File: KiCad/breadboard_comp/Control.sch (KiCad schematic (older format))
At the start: 88 parts, among them SW8 SW_Push, U2 74LS04, U57 74LS04, U85 74LS02, U87 74LS08, U88 74LS161, U89 74LS138, U90 28C256, U91 28C256, U92 74LS04, U93 28C256, U94 28C256, U95 74LS04, U96 74LS04

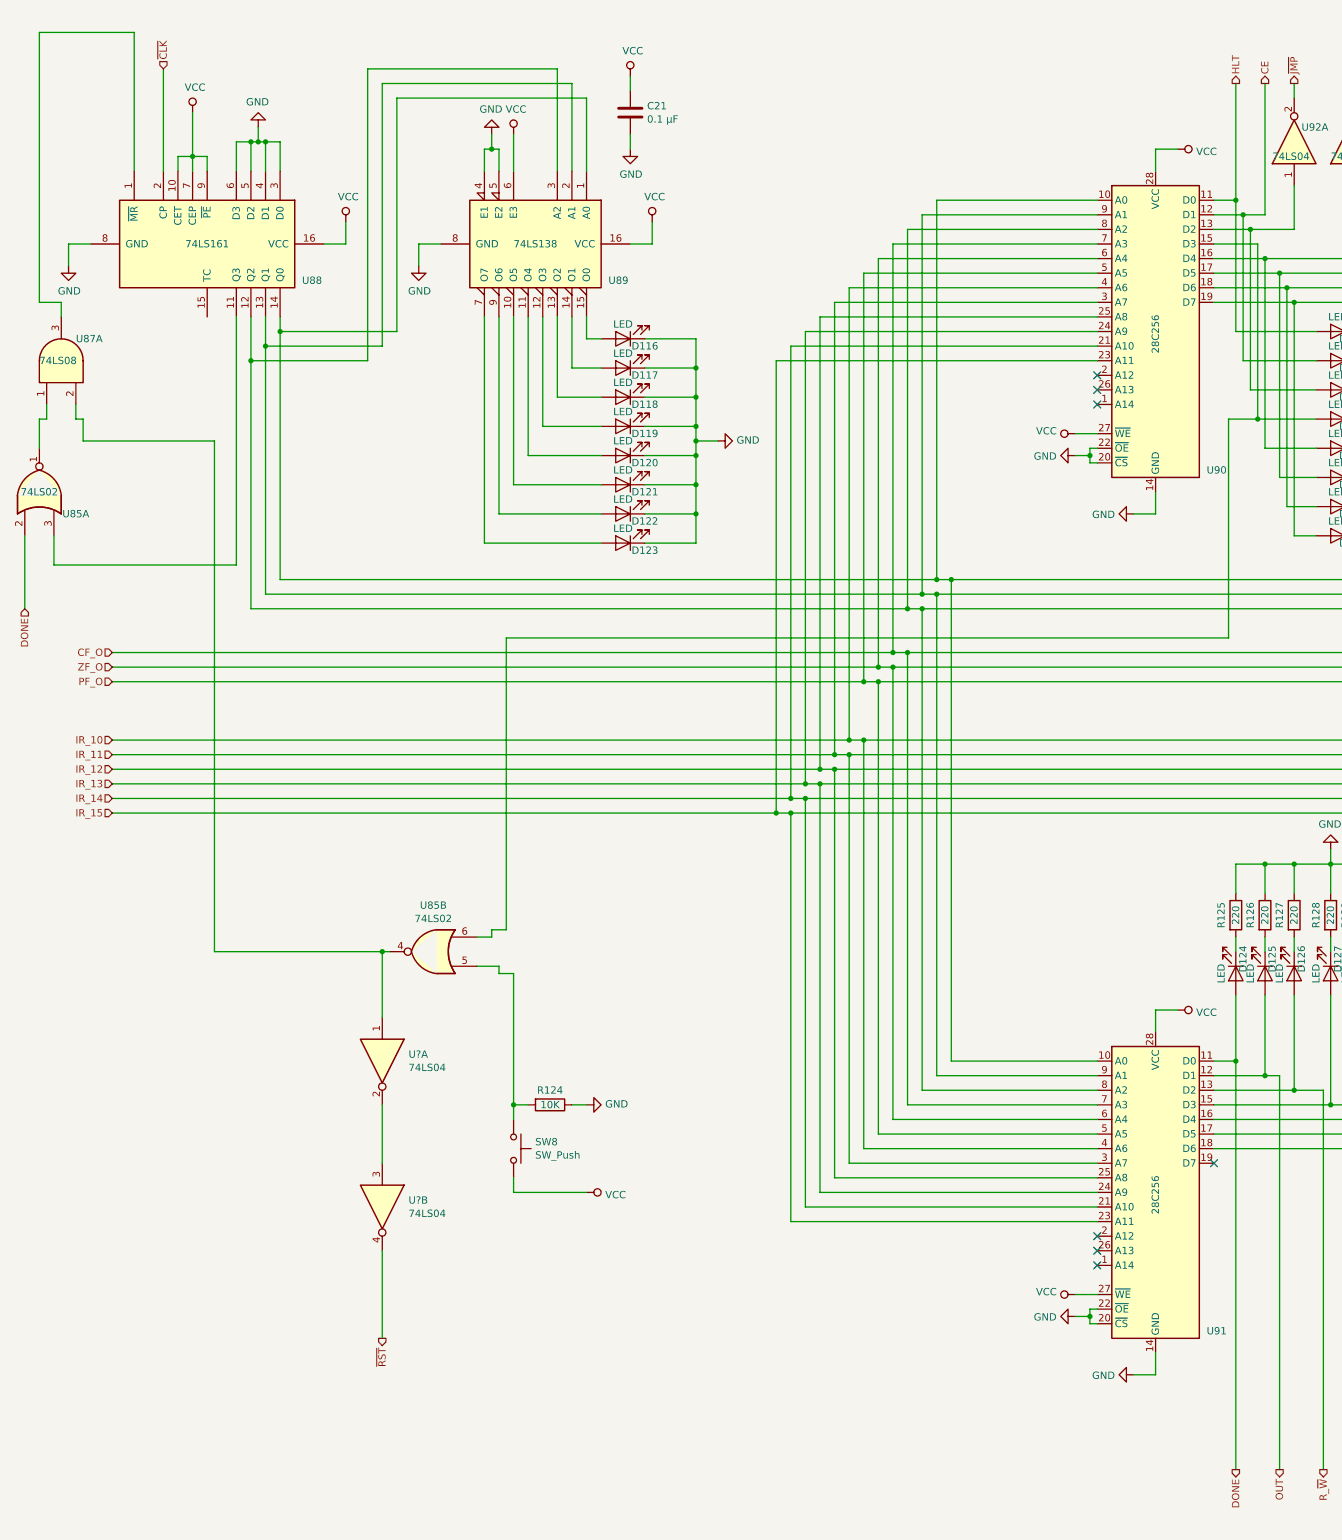
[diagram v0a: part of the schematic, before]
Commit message: Changes
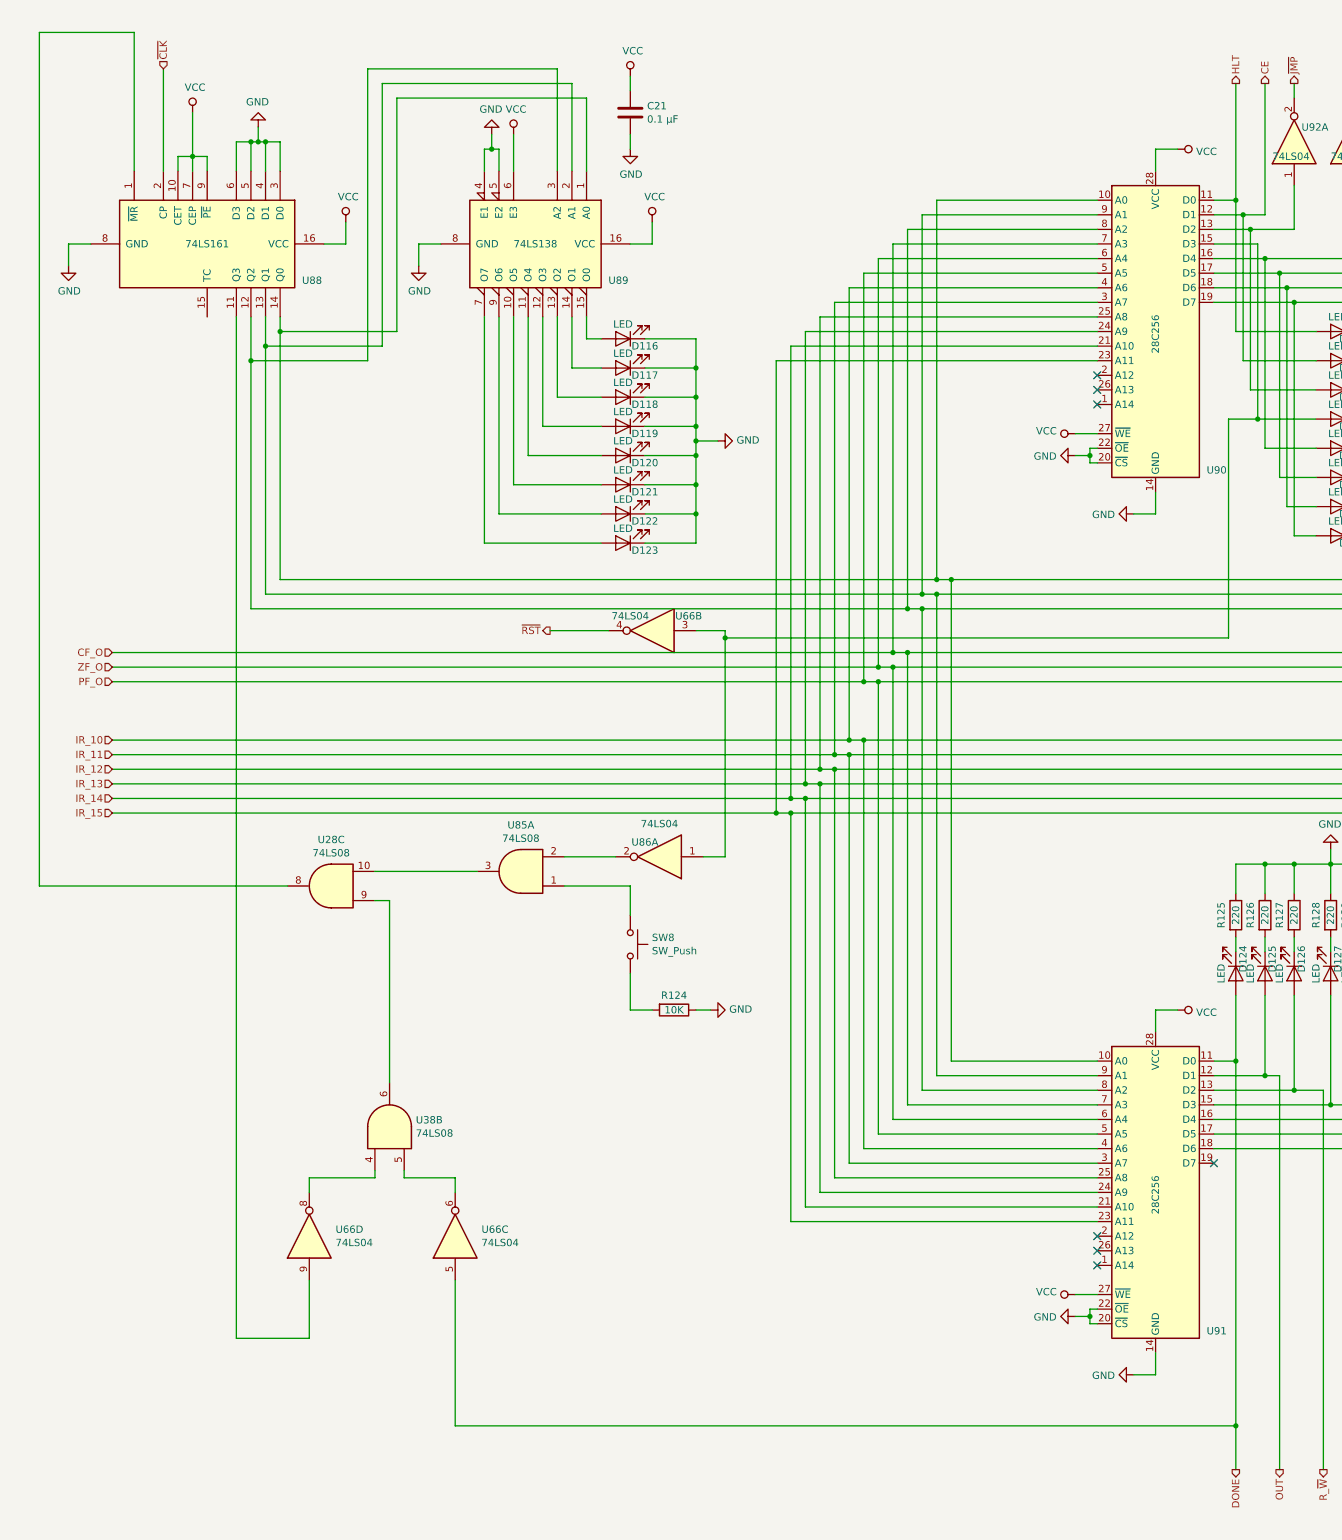
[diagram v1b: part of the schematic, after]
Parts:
- removed U85: 74LS02, symbol 74xx:74LS02
- removed U87: 74LS08, symbol 74xx:74LS08
- removed U? (x2): 74LS04, symbol 74xx:74LS04
- added U28, U38, U85: 74LS08, symbol 74xx:74LS08
- added U66, U86: 74LS04, symbol 74xx:74LS04
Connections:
- net DONE: now also U66.5
- net VCC: no longer SW8.2
- net ~RST: now also U66.4
- net at U88.1 (~MR): now also U28.8
- net at SW8.1: now also U85.1; no longer R124.2
- net at D131.2 (A), U90.15 (D3): now also U66.3, U86.1
- net at U88.11 (Q3): now also U66.9
- new net: R124.2, SW8.2
- new net: U85.2, U86.2
- new net: U28.10, U85.3
- new net: U38.5, U66.6
- new net: U38.4, U66.8
- new net: U28.9, U38.6
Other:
- moved on the sheet: R124, SW8
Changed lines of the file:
@@
 	10250 2450 10250 1650
-$Comp
-L 74xx:74LS08 U87
-U 1 1 5E950B6B
-P 800 2850
-F 0 "U87" V 950 2750 50  0000 R CNN
-F 1 "74LS08" V 800 3000 50  0000 R CNN
-F 2 "" H 800 2850 50  0001 C CNN
-F 3 "http://www.ti.com/lit/gpn/sn74LS08" H 800 2850 50  0001 C CNN
-	1    800  2850
-	0    -1   -1   0
-$EndComp
 $Comp
 L power:GND #PWR0218
@@
 $EndComp
 $Comp
-L 74xx:74LS02 U85
-U 1 1 5F5126B5
-P 650 3750
-F 0 "U85" V 500 3500 50  0000 C CNN
-F 1 "74LS02" V 650 3750 50  0000 C CNN
-F 2 "" H 650 3750 50  0001 C CNN
-F 3 "http://www.ti.com/lit/gpn/sn74ls02" H 650 3750 50  0001 C CNN
-	1    650  3750
-	0    -1   -1   0
-$EndComp
-$Comp
 L Switch:SW_Push SW8
 U 1 1 5E95E647
-P 3900 8250
-F 0 "SW8" V 3854 8398 50  0000 L CNN
-F 1 "SW_Push" V 3945 8398 50  0000 L CNN
-F 2 "" H 3900 8450 50  0001 C CNN
-F 3 "~" H 3900 8450 50  0001 C CNN
-	1    3900 8250
+P 4700 6850
+F 0 "SW8" V 4654 6998 50  0000 L CNN
+F 1 "SW_Push" V 4745 6998 50  0000 L CNN
+F 2 "" H 4700 7050 50  0001 C CNN
+F 3 "~" H 4700 7050 50  0001 C CNN
+	1    4700 6850
 	0    1    1    0
 $EndComp
@@
 L Device:R R124
 U 1 1 5E95EEBA
-P 4150 7950
-F 0 "R124" V 4050 7950 50  0000 C CNN
-F 1 "10K" V 4150 7950 50  0000 C CNN
-F 2 "" V 4080 7950 50  0001 C CNN
-F 3 "~" H 4150 7950 50  0001 C CNN
-	1    4150 7950
-	0    1    1    0
-$EndComp
-Wire Wire Line
-	3900 8550 3900 8450
-$Comp
-L power:VCC #PWR0219
-U 1 1 5E98986A
-P 4400 8550
-F 0 "#PWR0219" H 4400 8400 50  0001 C CNN
-F 1 "VCC" V 4417 8678 50  0000 L CNN
-F 2 "" H 4400 8550 50  0001 C CNN
-F 3 "" H 4400 8550 50  0001 C CNN
-	1    4400 8550
+P 5000 7300
+F 0 "R124" V 4900 7300 50  0000 C CNN
+F 1 "10K" V 5000 7300 50  0000 C CNN
+F 2 "" V 4930 7300 50  0001 C CNN
+F 3 "~" H 5000 7300 50  0001 C CNN
+	1    5000 7300
 	0    1    1    0
 $EndComp
@@
 L power:GND #PWR0220
 U 1 1 5E99EF31
-P 4400 7950
-F 0 "#PWR0220" H 4400 7700 50  0001 C CNN
-F 1 "GND" V 4405 7822 50  0000 R CNN
-F 2 "" H 4400 7950 50  0001 C CNN
-F 3 "" H 4400 7950 50  0001 C CNN
-	1    4400 7950
-	0    -1   -1   0
-$EndComp
-Wire Wire Line
-	4400 7950 4300 7950
-Wire Wire Line
-	650  3450 650  3250
-Wire Wire Line
-	650  3250 700  3250
-Wire Wire Line
-	700  3250 700  3150
-Wire Wire Line
-	800  2550 800  2450
-Wire Wire Line
-	800  2450 650  2450
-Wire Wire Line
-	650  600  650  2450
-Wire Wire Line
-	750  4050 750  4250
-Wire Wire Line
-	750  4250 2000 4250
-Wire Wire Line
-	2000 2550 2000 4250
+P 5250 7300
+F 0 "#PWR0220" H 5250 7050 50  0001 C CNN
+F 1 "GND" V 5255 7172 50  0000 R CNN
+F 2 "" H 5250 7300 50  0001 C CNN
+F 3 "" H 5250 7300 50  0001 C CNN
+	1    5250 7300
+	0    -1   -1   0
+$EndComp
+Wire Wire Line
+	5250 7300 5150 7300
 Text HLabel 15450 950  1    50   Output ~ 0
 ~AO
@@
 	8700 7650 8850 7650
 Wire Wire Line
-	8850 7650 8850 10450
+	8850 7650 8850 10150
 Wire Wire Line
 	9150 10450 9150 7750
@@
 Wire Wire Line
 	13350 9500 13350 9650
-Text HLabel 550  4550 3    50   Input ~ 0
-DONE
-Wire Wire Line
-	8800 4750 3850 4750
+Wire Wire Line
+	8800 4750 5350 4750
 $Comp
 L Device:LED D128
@@
 	0    -1   -1   0
 $EndComp
-Text HLabel 3000 9550 3    50   Output ~ 0
+Wire Wire Line
+	4850 7300 4700 7300
+Wire Wire Line
+	4700 7300 4700 7050
+$Comp
+L 74xx:74LS08 U85
+U 1 1 5EB8D5DD
+P 3950 6350
+F 0 "U85" H 3950 6033 50  0000 C CNN
+F 1 "74LS08" H 3950 6124 50  0000 C CNN
+F 2 "" H 3950 6350 50  0001 C CNN
+F 3 "http://www.ti.com/lit/gpn/sn74LS08" H 3950 6350 50  0001 C CNN
+	1    3950 6350
+	-1   0    0    1
+$EndComp
+$Comp
+L 74xx:74LS04 U86
+U 1 1 5EB92E4C
+P 4900 6250
+F 0 "U86" H 5000 6150 50  0000 C CNN
+F 1 "74LS04" H 4900 6024 50  0000 C CNN
+F 2 "" H 4900 6250 50  0001 C CNN
+F 3 "http://www.ti.com/lit/gpn/sn74LS04" H 4900 6250 50  0001 C CNN
+	1    4900 6250
+	-1   0    0    1
+$EndComp
+Wire Wire Line
+	5200 6250 5350 6250
+Wire Wire Line
+	5350 6250 5350 4750
+$Comp
+L 74xx:74LS04 U66
+U 2 1 5EBCD1CB
+P 4850 4700
+F 0 "U66" H 4600 4600 50  0000 C CNN
+F 1 "74LS04" H 5000 4600 50  0000 C CNN
+F 2 "" H 4850 4700 50  0001 C CNN
+F 3 "http://www.ti.com/lit/gpn/sn74LS04" H 4850 4700 50  0001 C CNN
+	2    4850 4700
+	-1   0    0    1
+$EndComp
+Wire Wire Line
+	5350 4750 5350 4700
+Wire Wire Line
+	5350 4700 5150 4700
+Connection ~ 5350 4750
+Text HLabel 4150 4700 0    50   Output ~ 0
 ~RST
 Wire Wire Line
-	1850 6900 1850 3400
-Wire Wire Line
-	1850 3400 950  3400
-Wire Wire Line
-	950  3400 950  3250
-Wire Wire Line
-	950  3250 900  3250
-Wire Wire Line
-	900  3250 900  3150
-Wire Wire Line
-	550  4050 550  4550
-$Comp
-L 74xx:74LS02 U85
-U 2 1 5EE72376
-P 3350 6900
-F 0 "U85" H 3350 6583 50  0000 C CNN
-F 1 "74LS02" H 3350 6674 50  0000 C CNN
-F 2 "" H 3350 6900 50  0001 C CNN
-F 3 "http://www.ti.com/lit/gpn/sn74ls02" H 3350 6900 50  0001 C CNN
-	2    3350 6900
-	-1   0    0    1
-$EndComp
-Wire Wire Line
-	3850 6750 3750 6750
-Wire Wire Line
-	3750 6750 3750 6800
-Wire Wire Line
-	3750 6800 3650 6800
-Wire Wire Line
-	3850 4750 3850 6750
-Wire Wire Line
-	3900 7050 3800 7050
-Wire Wire Line
-	3800 7050 3800 7000
-Wire Wire Line
-	3800 7000 3650 7000
-Wire Wire Line
-	3900 7050 3900 7950
-Wire Wire Line
-	4000 7950 3900 7950
-Connection ~ 3900 7950
-Wire Wire Line
-	3900 7950 3900 8050
-Wire Wire Line
-	3900 8550 4400 8550
-Wire Wire Line
-	3050 6900 3000 6900
-Connection ~ 3000 6900
-Wire Wire Line
-	1850 6900 3000 6900
-$Comp
-L 74xx:74LS04 U?
-U 1 1 5EA8906A
-P 3000 7650
-F 0 "U?" V 2954 7830 50  0000 L CNN
-F 1 "74LS04" V 3045 7830 50  0000 L CNN
-F 2 "" H 3000 7650 50  0001 C CNN
-F 3 "http://www.ti.com/lit/gpn/sn74LS04" H 3000 7650 50  0001 C CNN
-	1    3000 7650
-	0    1    1    0
-$EndComp
-$Comp
-L 74xx:74LS04 U?
-U 2 1 5EA8A0BB
-P 3000 8650
-F 0 "U?" V 2954 8830 50  0000 L CNN
-F 1 "74LS04" V 3045 8830 50  0000 L CNN
-F 2 "" H 3000 8650 50  0001 C CNN
-F 3 "http://www.ti.com/lit/gpn/sn74LS04" H 3000 8650 50  0001 C CNN
-	2    3000 8650
-	0    1    1    0
-$EndComp
-Wire Wire Line
-	3000 9550 3000 8950
-Wire Wire Line
-	3000 8350 3000 7950
-Wire Wire Line
-	3000 6900 3000 7350
+	4150 4700 4550 4700
+Wire Wire Line
+	4700 6650 4700 6450
+Wire Wire Line
+	4700 6450 4250 6450
+Wire Wire Line
+	4250 6250 4600 6250
+$Comp
+L 74xx:74LS04 U66
+U 3 1 5ECF4F38
+P 3500 8850
+F 0 "U66" V 3546 8670 50  0000 R CNN
+F 1 "74LS04" V 3455 8670 50  0000 R CNN
+F 2 "" H 3500 8850 50  0001 C CNN
+F 3 "http://www.ti.com/lit/gpn/sn74LS04" H 3500 8850 50  0001 C CNN
+	3    3500 8850
+	0    -1   -1   0
+$EndComp
+$Comp
+L 74xx:74LS04 U66
+U 4 1 5ECF613E
+P 2500 8850
+F 0 "U66" V 2546 8670 50  0000 R CNN
+F 1 "74LS04" V 2455 8670 50  0000 R CNN
+F 2 "" H 2500 8850 50  0001 C CNN
+F 3 "http://www.ti.com/lit/gpn/sn74LS04" H 2500 8850 50  0001 C CNN
+	4    2500 8850
+	0    -1   -1   0
+$EndComp
+Wire Wire Line
+	2000 9550 2500 9550
+Wire Wire Line
+	2500 9550 2500 9150
+Wire Wire Line
+	2000 2550 2000 9550
+Wire Wire Line
+	3500 9150 3500 10150
+Wire Wire Line
+	3500 10150 8850 10150
+Connection ~ 8850 10150
+Wire Wire Line
+	8850 10150 8850 10450
+$Comp
+L 74xx:74LS08 U38
+U 2 1 5ED709EA
+P 3050 8100
+F 0 "U38" V 3096 7920 50  0000 R CNN
+F 1 "74LS08" V 3005 7920 50  0000 R CNN
+F 2 "" H 3050 8100 50  0001 C CNN
+F 3 "http://www.ti.com/lit/gpn/sn74LS08" H 3050 8100 50  0001 C CNN
+	2    3050 8100
+	0    -1   -1   0
+$EndComp
+Wire Wire Line
+	3150 8400 3150 8450
+Wire Wire Line
+	3150 8450 3500 8450
+Wire Wire Line
+	3500 8450 3500 8550
+Wire Wire Line
+	2500 8550 2500 8450
+Wire Wire Line
+	2500 8450 2950 8450
+Wire Wire Line
+	2950 8450 2950 8400
+$Comp
+L 74xx:74LS08 U28
+U 3 1 5EDEEB08
+P 2650 6450
+F 0 "U28" H 2650 6133 50  0000 C CNN
+F 1 "74LS08" H 2650 6224 50  0000 C CNN
+F 2 "" H 2650 6450 50  0001 C CNN
+F 3 "http://www.ti.com/lit/gpn/sn74LS08" H 2650 6450 50  0001 C CNN
+	3    2650 6450
+	-1   0    0    1
+$EndComp
+Wire Wire Line
+	2950 6350 3650 6350
+Wire Wire Line
+	3050 7800 3050 6550
+Wire Wire Line
+	3050 6550 2950 6550
+Wire Wire Line
+	2350 6450 650  6450
+Wire Wire Line
+	650  600  650  6450
 $EndSCHEMATC
